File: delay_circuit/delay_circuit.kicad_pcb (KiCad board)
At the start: 2 copper layers, 133 x 90 mm, 26 parts, among them J1 IN 12V AC, J2 OUT 230V AC, J3 IN 230V AC, J4 From Trfo Output, J5 OUT 5V CC, J6 To Power Ampli Power IN, J7 From Ampli Output, J8 OUT 12V CC, J9 To Speakers, K1 SANYOU_SRD_Form_C, K2 SANYOU_SRD_Form_C, Q1 NPN, Q2 NPN, U1 LM7812_TO220

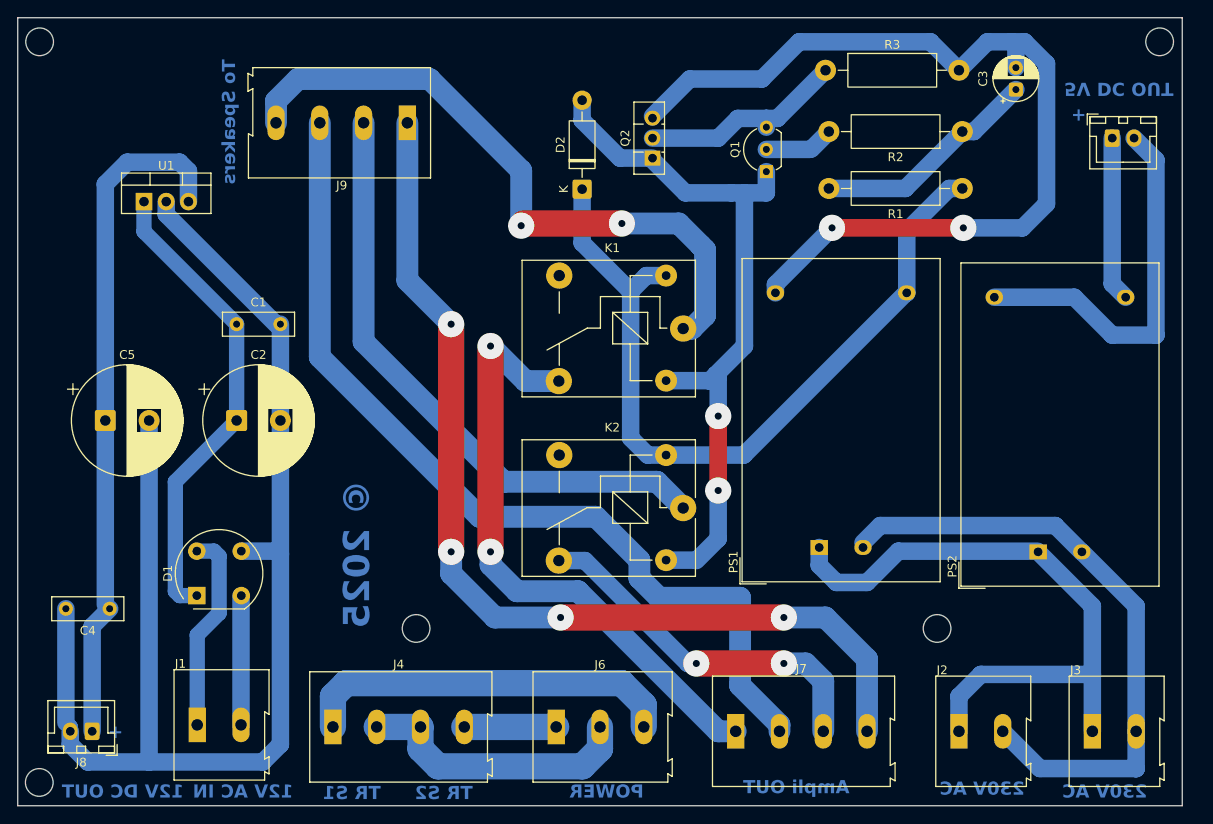
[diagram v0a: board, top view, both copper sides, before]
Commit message: Improved board.
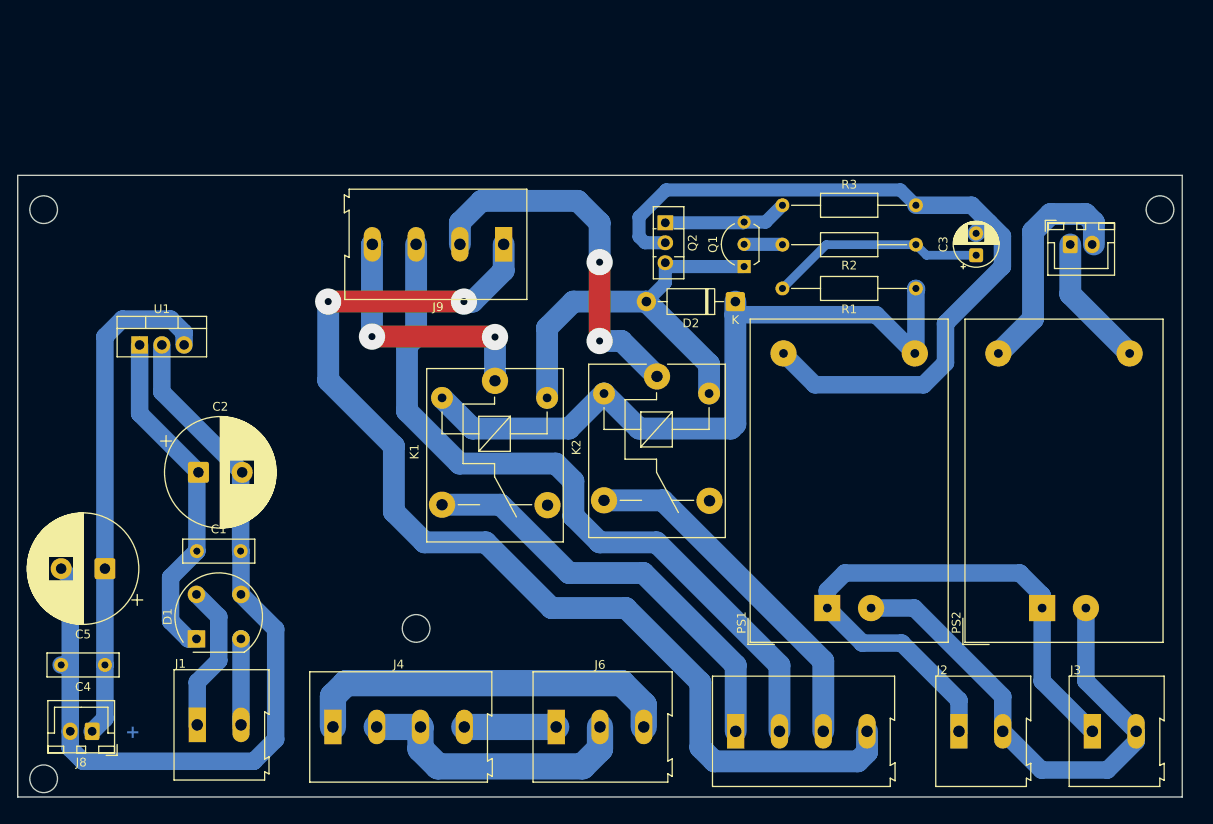
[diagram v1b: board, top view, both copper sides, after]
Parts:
- PS1, PS2: footprint Converter_ACDC:Converter_ACDC_Hi-Link_HLK-PMxx -> Components:Converter_ACDC_Hi-Link_HLK-PMxx
- Q2: footprint Package_TO_SOT_THT:TO-126-3_Vertical -> Components:TO-126-3_Vertical
- R1, R2, R3: footprint Resistor_THT:R_Axial_DIN0411_L9.9mm_D3.6mm_P15.24mm_Horizontal -> Resistor_THT:R_Axial_DIN0207_L6.3mm_D2.5mm_P15.24mm_Horizontal
- moved C1 26.3 mm to (55.0, 86.0)
- moved K1 22.3 mm to (89.0, 66.5), turned to -90 degrees
- moved D2 21.7 mm to (116.5, 57.5), turned to 180 degrees
- moved C3 19.5 mm to (144.0, 52.2)
- moved J9 17.7 mm to (90.0, 51.0)
- moved C5 16.9 mm to (44.5, 88.0), turned to 180 degrees
- moved U1 16.4 mm to (48.5, 62.5)
- moved R3 16.2 mm to (121.9, 46.5)
- moved K2 15.3 mm to (107.5, 66.0), turned to -90 degrees
- moved R2 14.0 mm to (137.1, 51.0)
- moved J5 13.1 mm to (154.8, 51.0)
- moved R1 12.6 mm to (137.1, 56.0)
- moved Q1 11.1 mm to (117.5, 53.5)
- moved Q2 7.53 mm to (108.5, 48.5), turned to -90 degrees
- moved C2 7.35 mm to (55.2, 77.0)
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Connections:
- K1 pad 3: unconnected-(K1-Pad3) -> IN SP L+
- K1 pad 4: IN SP L+ -> unconnected-(K1-Pad4)
- K2 pad 3: unconnected-(K2-Pad3) -> IN SP R+
- K2 pad 4: IN SP R+ -> unconnected-(K2-Pad4)
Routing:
- net 12V GND: track 152.7 -> 97.7 mm
- net OUT SP L+: track 75.1 -> 29.6 mm
- net Net-(D2-A): track 83.1 -> 48.6 mm, vias 2 -> 0
- net OUT SP R+: track 69.4 -> 42.2 mm, vias 0 -> 2
- net IN SP L+: track 70.3 -> 48.7 mm, vias 2 -> 0
- net Net-(J7-Pin_2): track 104.4 -> 83.9 mm
- net Net-(J8-Pin_1): track 78.0 -> 57.6 mm
- net Net-(J5-Pin_2): track 43.8 -> 26.3 mm
- net 0: track 107.4 -> 91.3 mm, vias 2 -> 0
- net Net-(D1-+): track 54.4 -> 39.4 mm
- net Net-(J2-Pin_2): track 71.9 -> 59.2 mm
- net Net-(J7-Pin_4): track 113.4 -> 124.7 mm, vias 4 -> 2
- net Net-(Q1-E): track 24.0 -> 14.2 mm
- net Net-(D2-K): track 91.0 -> 82.4 mm
- net Net-(J1-Pin_1): track 23.1 -> 17.0 mm
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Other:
- board size 133 x 90 mm -> 133 x 71 mm
- board text removed: "12V AC IN"
- board text removed: "12V DC OUT"
- board text removed: "230V AC"
- board text removed: "5V DC OUT"
- board text removed: "Ampli OUT"
- board text removed: "POWER"
- board text removed: "TR S1"
- board text removed: "TR S2"
- board text removed: "To Speakers"
- board text removed: "© 2025"
